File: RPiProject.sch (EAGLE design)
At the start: 26 parts

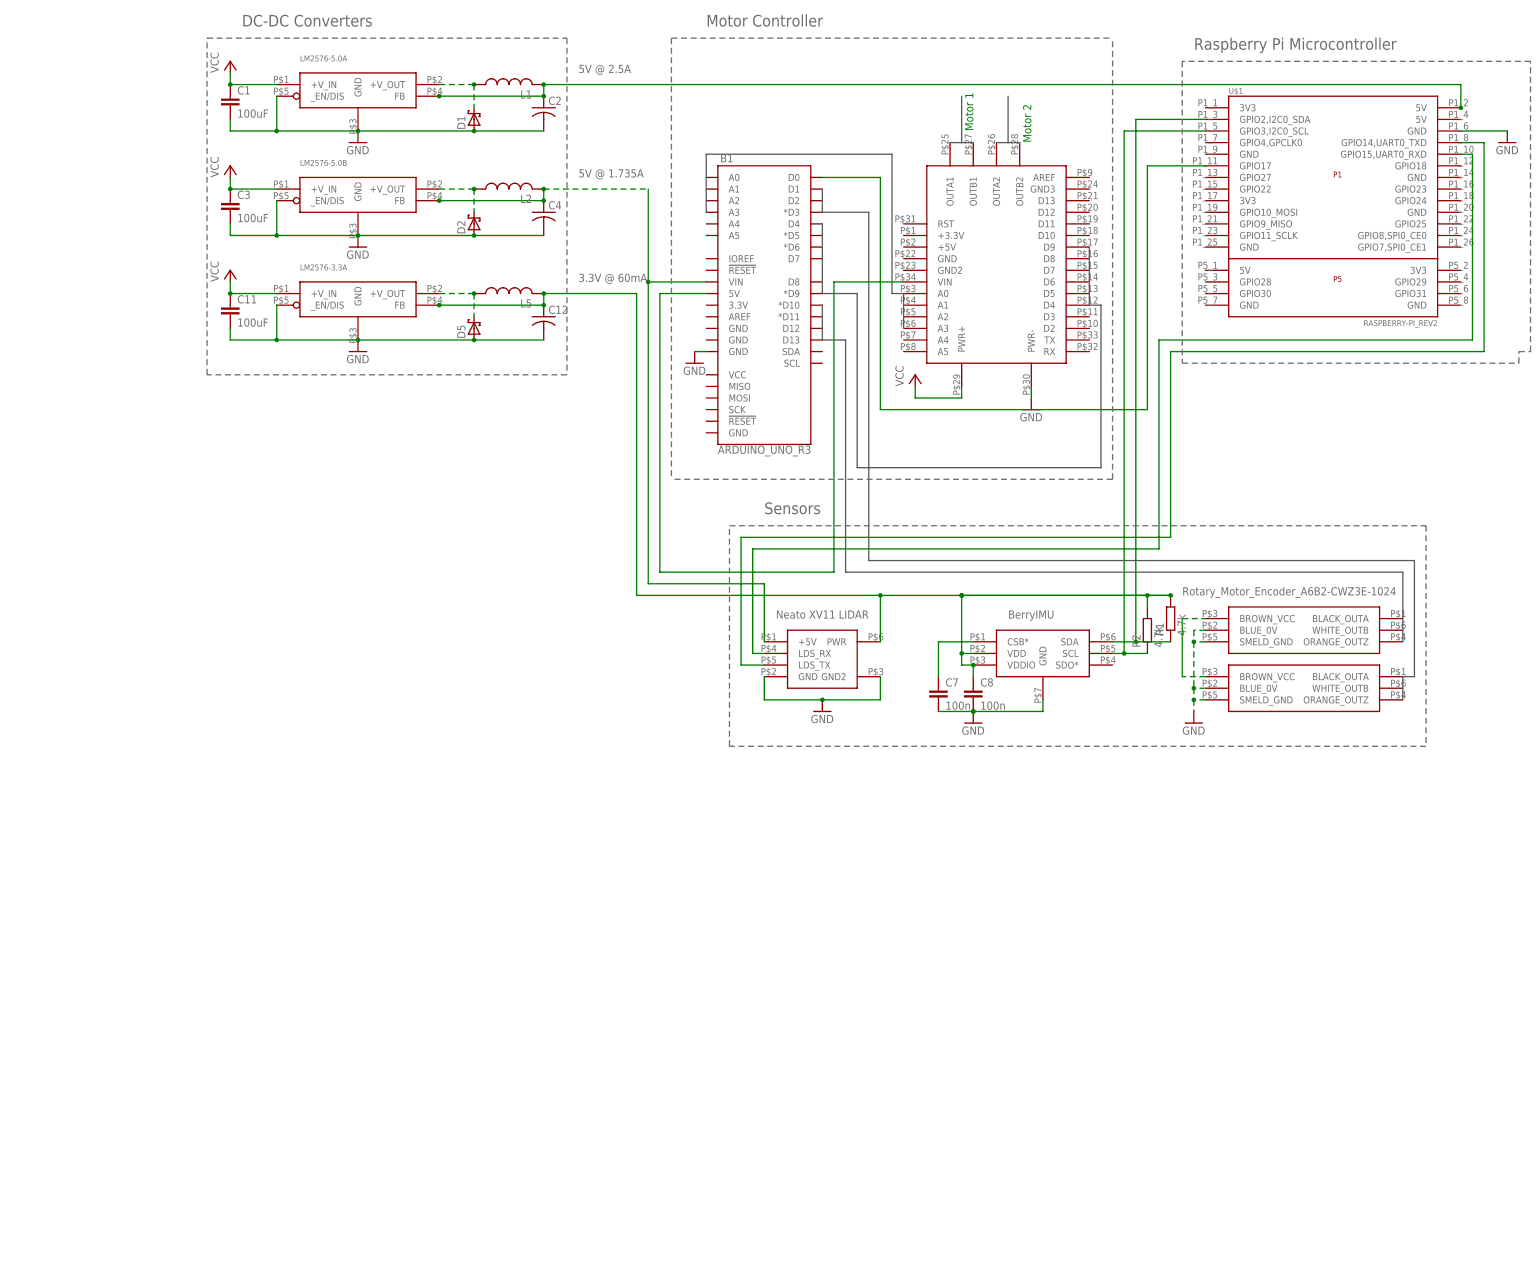
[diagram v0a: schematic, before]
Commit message: Updated motor controller
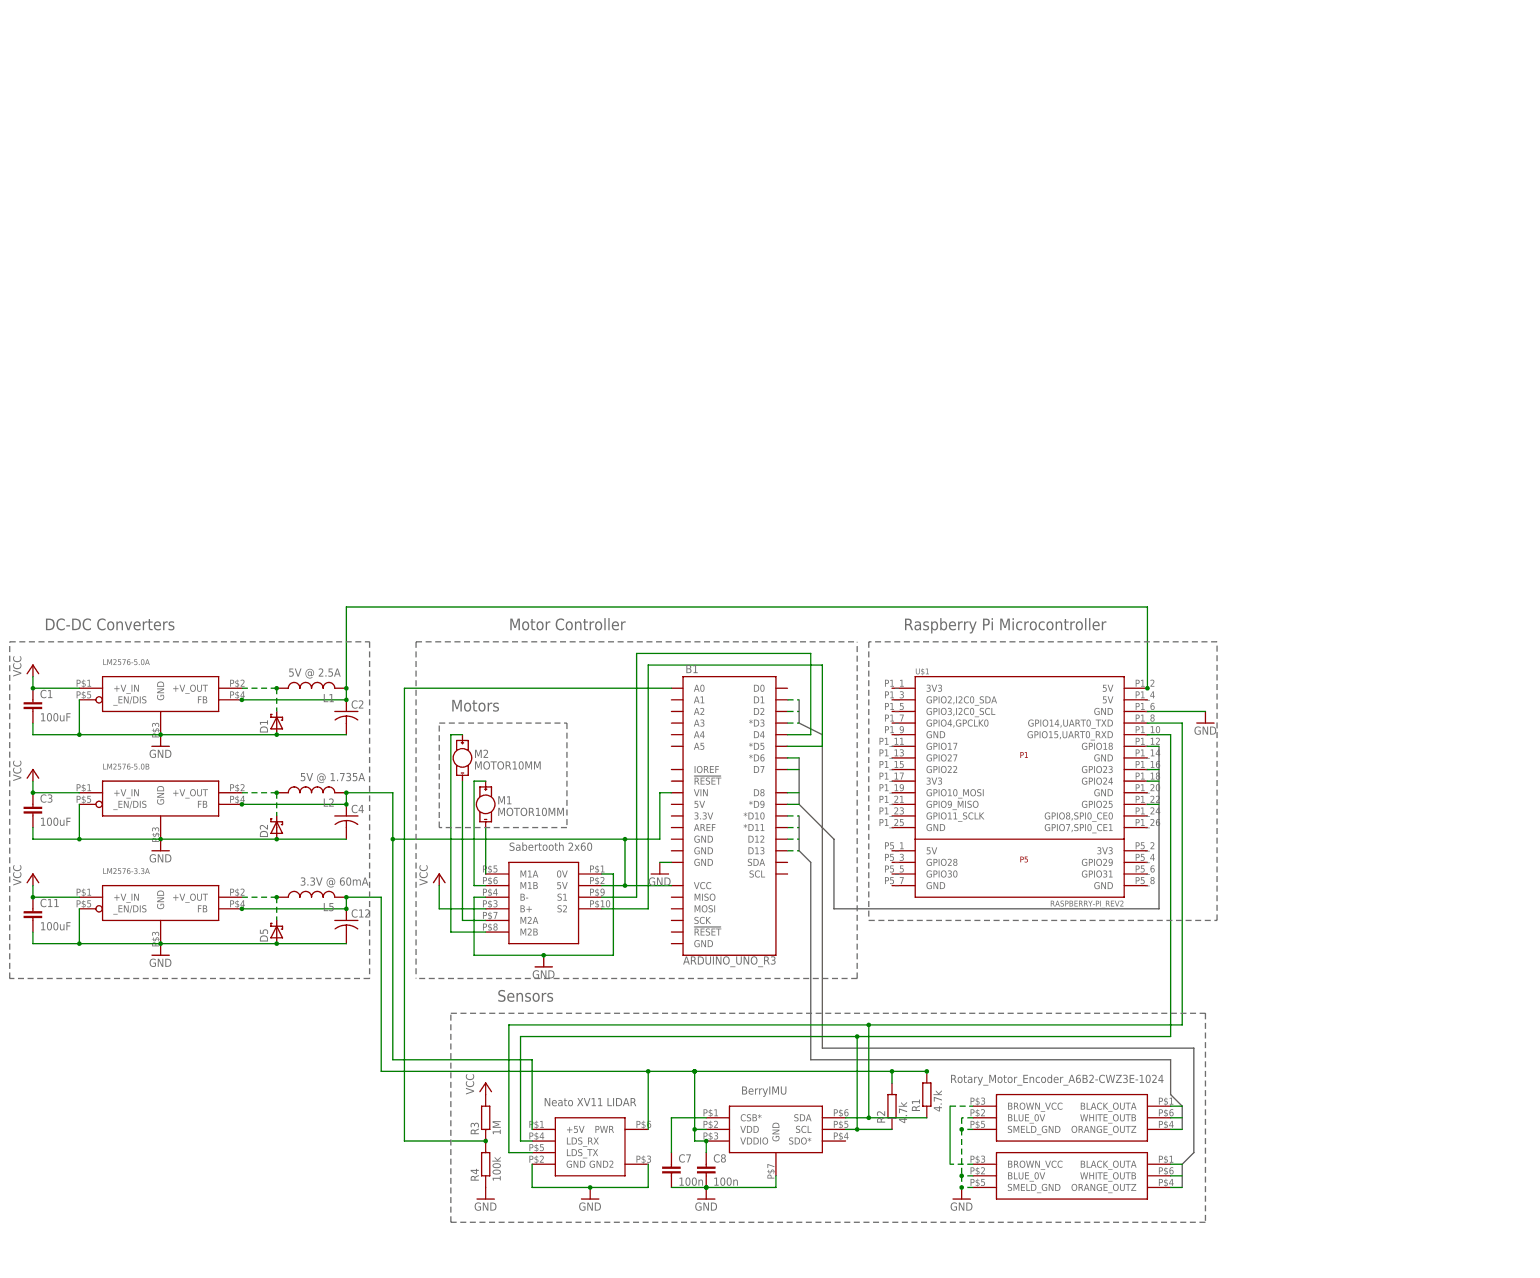
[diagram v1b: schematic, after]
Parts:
- removed U$5: MONSTERMOTO, RaspberryPi:MONSTERMOTO
- added M1, M2: MOTOR10MM, SparkFun-Electromechanical:MOTOR10MM
- added R3: 1M, ee2parts:R
- added R4: 100k, ee2parts:R
- added U$6: SABERTOOTH2X60, RaspberryPi:SABERTOOTH2X60
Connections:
- removed net N$15: U$1.GPIO14,UART0_TXD, XV11LIDAR.LDS_TX
- removed net N$16: B1.D0, U$1.GPIO17
- new net B$1: B1.*D10, B1.*D11, B1.D12, B1.D13, U$2.BLACK_OUTA, U$2.ORANGE_OUTZ, U$2.WHITE_OUTB
- new net B$2: B1.*D6, B1.*D9, B1.D7, B1.D8, U$1.GPIO18, U$1.GPIO23, U$1.GPIO24, U$1.GPIO25
- new net B$4: B1.*D3, B1.D1, B1.D2, U$3.BLACK_OUTA, U$3.ORANGE_OUTZ, U$3.WHITE_OUTB
- new net N$13: M1.+, U$6.M1B
- new net N$14: R2.1, U$1.GPIO15,UART0_RXD, U$4.SCL, XV11LIDAR.LDS_RX
- new net N$23: B1.VCC, B1.VIN, C4.1, L2.2, LM2576-5.0B.FB, U$6.5V, XV11LIDAR.+5V
- new net N$4: B1.A0, R3.1, R4.2
- new net N$8: B1.D4, U$6.S1
- net GND: now also R4.1, U$6.0V, U$6.B-; no longer U$5.PWR-
- net N$1: now also M2.+, U$6.M2B; no longer B1.5V, U$5.VIN
- net N$10: now also U$1.GPIO14,UART0_TXD, XV11LIDAR.LDS_TX; no longer U$1.GPIO2,I2C0_SDA
- net N$17: now also B1.*D5, U$6.S2; no longer U$1.GPIO15,UART0_RXD, XV11LIDAR.LDS_RX
- net N$7: now also M2.-, U$6.M2A; no longer B1.VIN, C4.1, L2.2, LM2576-5.0B.FB, XV11LIDAR.+5V
- net N$9: now also M1.-, U$6.M1A; no longer R2.1, U$1.GPIO3,I2C0_SCL, U$4.SCL
- net VCC: now also R3.2, U$6.B+; no longer U$5.PWR+
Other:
- note added: "Motors"
- note added: "Sabertooth 2x60"
- note removed: "Motor 1"
- note removed: "Motor 2"
- moved on the sheet: B1, C1, C11, C12, C2, C3, C4, C7, C8, D1, D2, D5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

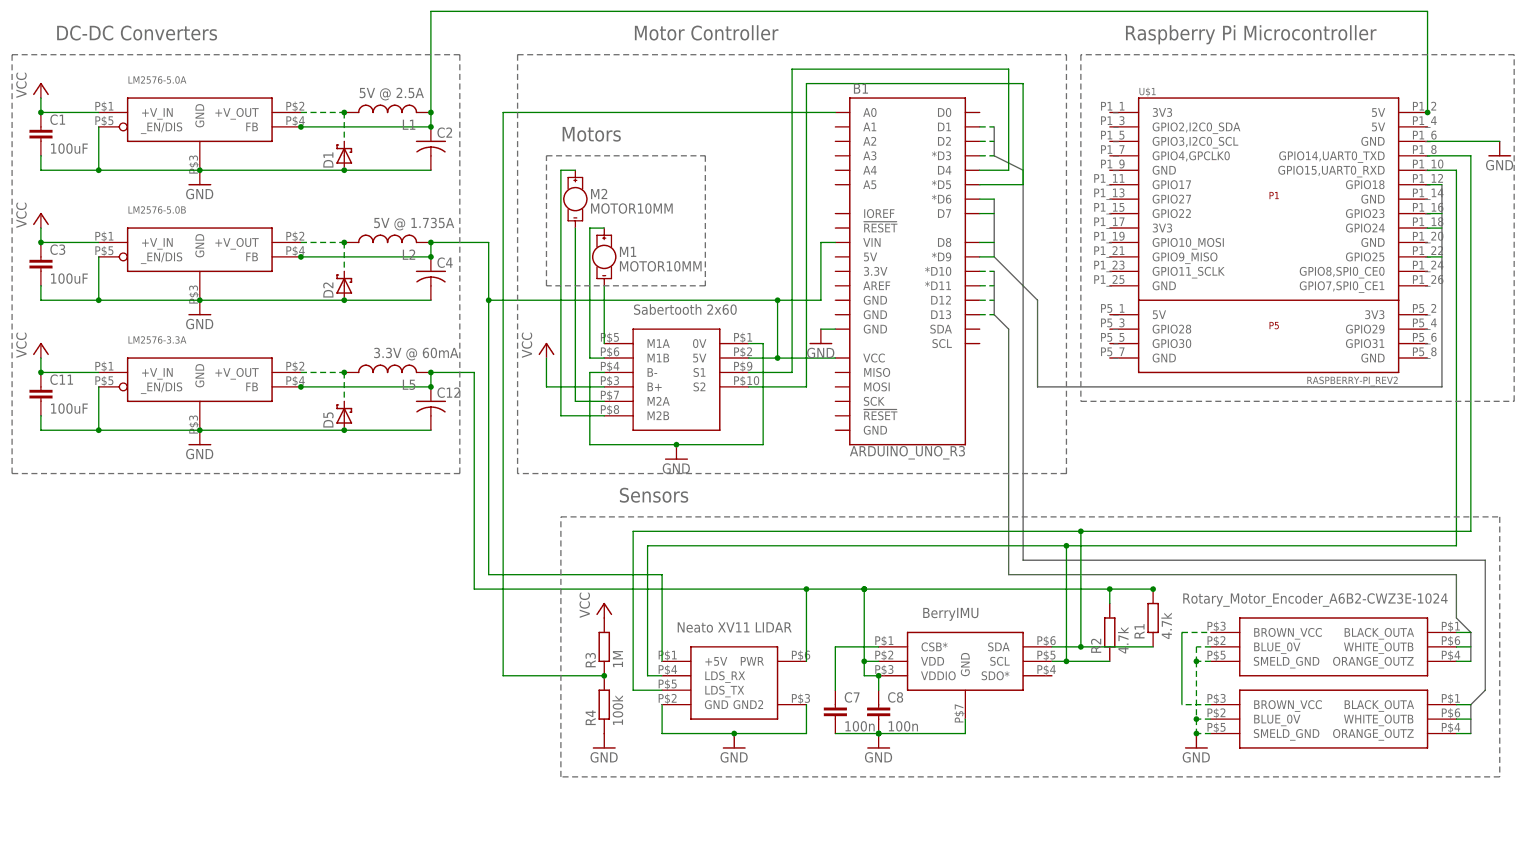
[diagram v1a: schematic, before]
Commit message: Updated arduino pin layout
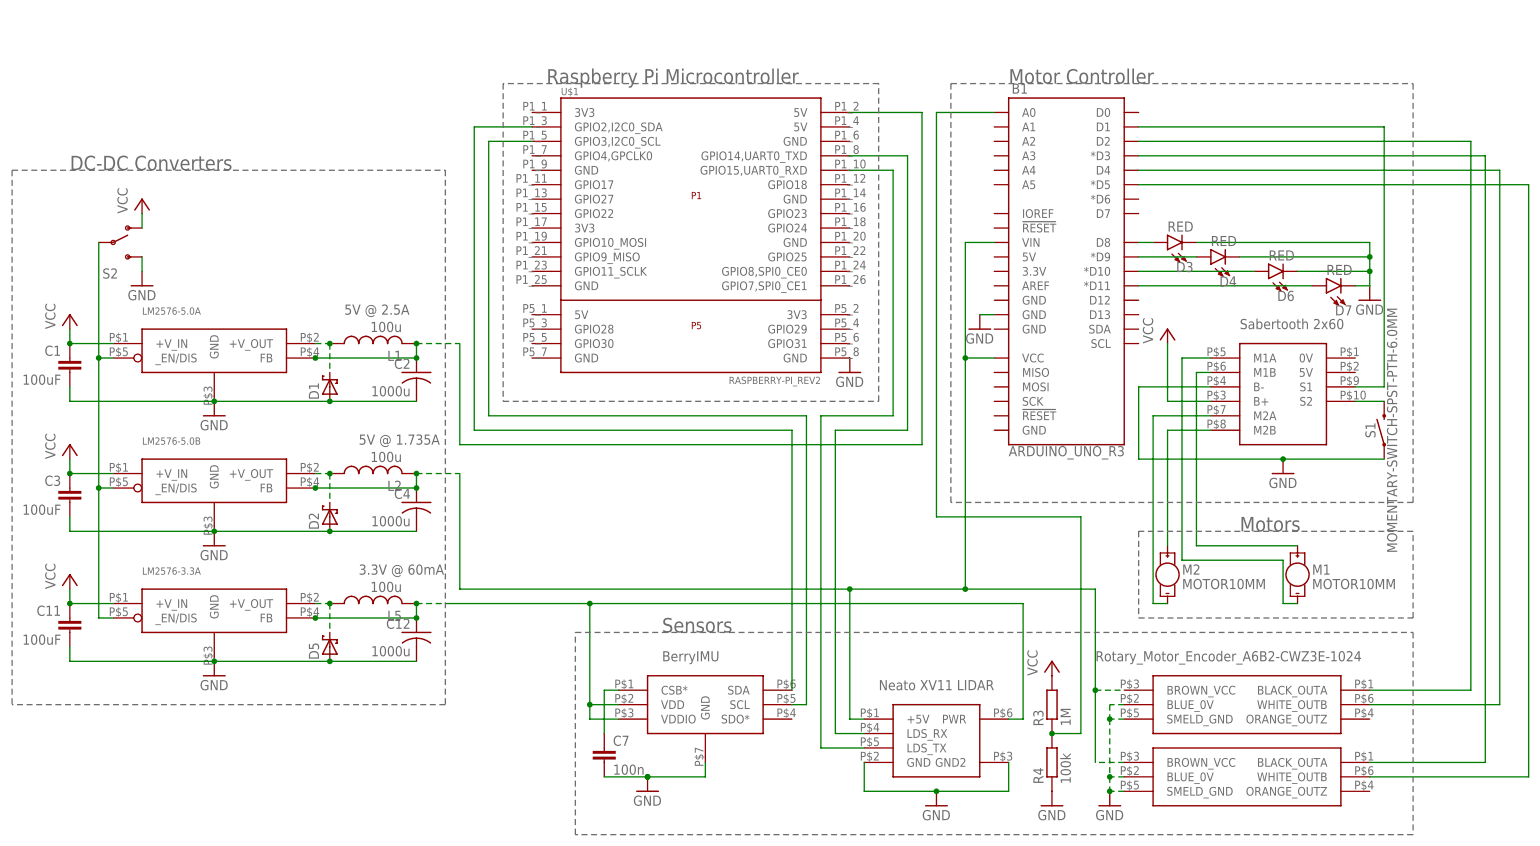
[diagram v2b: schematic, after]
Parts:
- removed C8: 100n, ee2parts:C2.5P
- removed R1, R2: 4.7k, ee2parts:R
- added D3, D4, D6, D7: RED, SparkFun-LED:LED-RED0603
- added S1: MOMENTARY-SWITCH-SPST-PTH-6.0MM, SparkFun-Switches:MOMENTARY-SWITCH-SPST-PTH-6.0MM
- added S2: (no value), SparkFun-Retired:SWITCH-SPDTPTH2
- C12, C2, C4: value (none) -> 1000u
- L1, L2, L5: value (none) -> 100u
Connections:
- removed net B$1: B1.*D10, B1.*D11, B1.D12, B1.D13, U$2.BLACK_OUTA, U$2.ORANGE_OUTZ, U$2.WHITE_OUTB
- removed net B$2: B1.*D6, B1.*D9, B1.D7, B1.D8, U$1.GPIO18, U$1.GPIO23, U$1.GPIO24, U$1.GPIO25
- removed net B$4: B1.*D3, B1.D1, B1.D2, U$3.BLACK_OUTA, U$3.ORANGE_OUTZ, U$3.WHITE_OUTB
- removed net N$14: R2.1, U$1.GPIO15,UART0_RXD, U$4.SCL, XV11LIDAR.LDS_RX
- removed net N$8 (its old number): B1.D4, U$6.S1
- new net N$12: U$1.GPIO3,I2C0_SCL, U$4.SCL
- new net N$15: U$1.GPIO2,I2C0_SDA, U$4.SDA
- new net N$19: B1.*D3, U$3.BLACK_OUTA
- new net N$21: B1.*D5, U$3.WHITE_OUTB
- new net N$22: B1.D4, U$2.WHITE_OUTB
- new net N$25: LM2576-3.3A._EN/DIS, LM2576-5.0A._EN/DIS, LM2576-5.0B._EN/DIS, S2.P
- new net N$26: U$1.GPIO15,UART0_RXD, XV11LIDAR.LDS_TX
- new net N$27: B1.*D9, D4.A
- new net N$28: B1.*D10, D6.A
- new net N$29: B1.*D11, D7.A
- new net N$3: B1.D1, U$6.S1
- new net N$30: D3.C, D4.C, D6.C, D7.C
- new net N$9: B1.D8, D3.A
- net GND: now also B1.GND@1, S1.1, S2.S, U$1.GND@P5_8; no longer B1.GND@0, C8.2, U$1.GND@6, U$6.0V
- net GND2: no longer LM2576-3.3A._EN/DIS, LM2576-5.0A._EN/DIS, LM2576-5.0B._EN/DIS
- net N$10: now also XV11LIDAR.LDS_RX; no longer R1.1, U$4.SDA, XV11LIDAR.LDS_TX
- net N$11: now also B1.D2, U$2.BLACK_OUTA; no longer U$2.BROWN_VCC, U$3.BROWN_VCC
- net N$17: now also S1.2; no longer B1.*D5
- net N$23: now also U$2.BROWN_VCC, U$3.BROWN_VCC; no longer U$6.5V
- net N$5: no longer C8.1, R1.2, R2.2
- net VCC: now also S2.O
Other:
- moved on the sheet: B1, C1, C11, C12, C2, C3, C4, C7, D1, D2, D5, L1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
